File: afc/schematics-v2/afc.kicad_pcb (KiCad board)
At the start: 2 copper layers, 116.8 x 67.3 mm, 16 parts

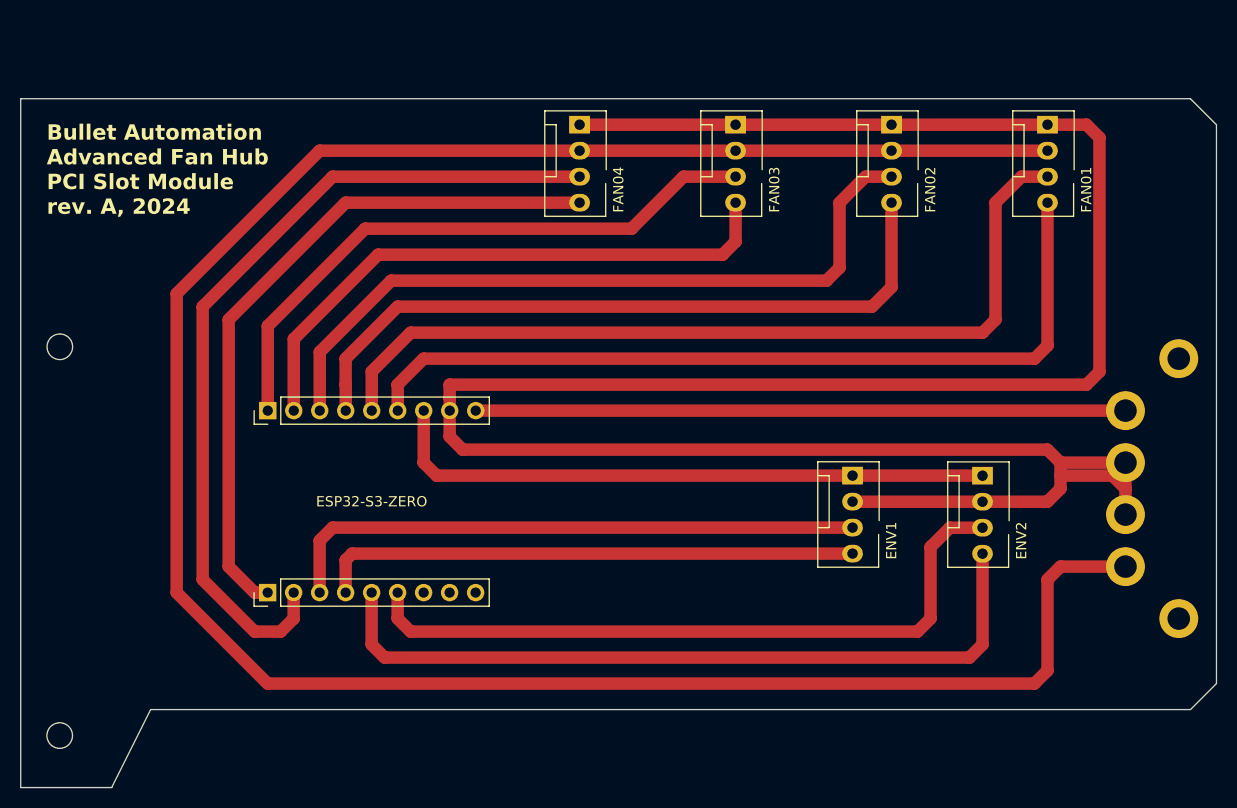
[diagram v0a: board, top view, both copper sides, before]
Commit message: adding v2 schematics
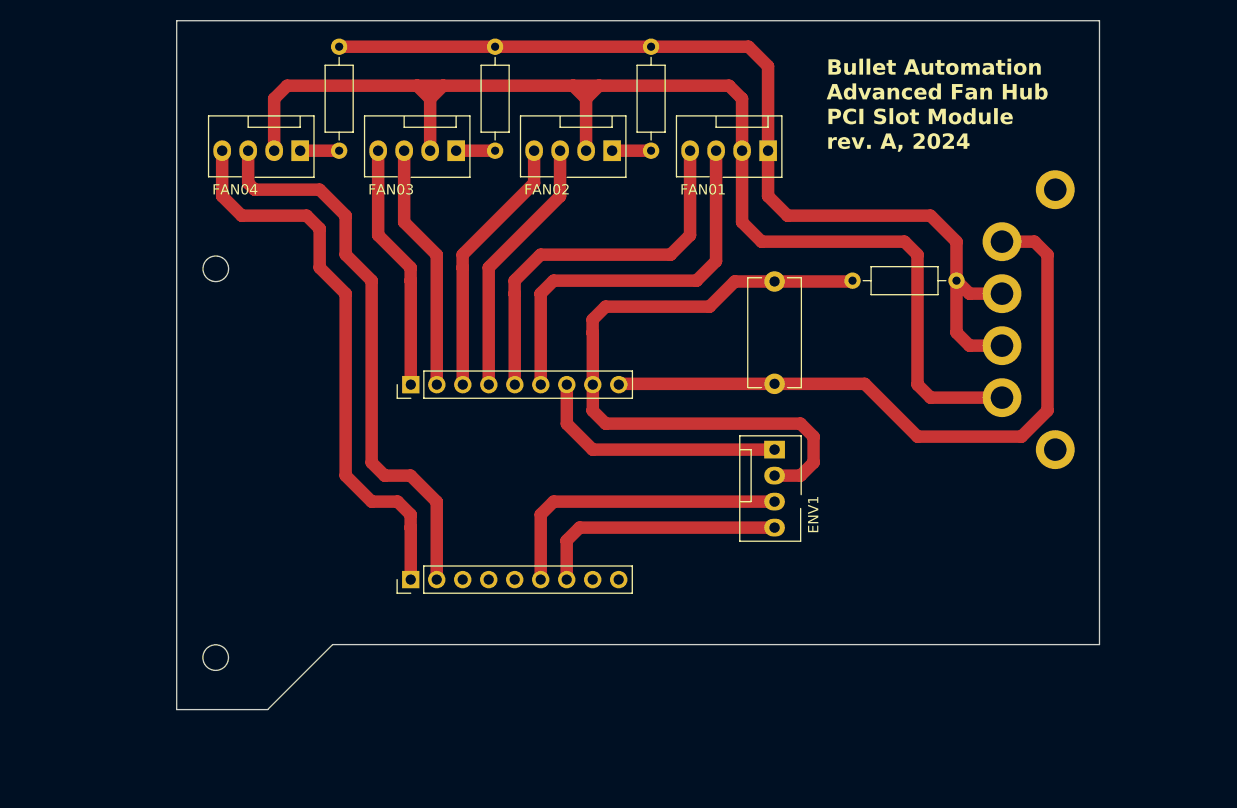
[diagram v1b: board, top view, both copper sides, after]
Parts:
- removed ENV2: FAN_H4, Connector:FanPinHeader_1x04_P2.54mm_Vertical
- added Ce: C_Disc_D10.5mm_W5.0mm_P10.00mm, Capacitor_THT:C_Disc_D10.5mm_W5.0mm_P10.00mm, F.Cu at (162.6, 87.5)
- added REF**: R_Axial_DIN0207_L6.3mm_D2.5mm_P10.16mm_Horizontal, Resistor_THT:R_Axial_DIN0207_L6.3mm_D2.5mm_P10.16mm_Horizontal, F.Cu at (135.3, 54.6)
- added REF**: R_Axial_DIN0207_L6.3mm_D2.5mm_P10.16mm_Horizontal, Resistor_THT:R_Axial_DIN0207_L6.3mm_D2.5mm_P10.16mm_Horizontal, F.Cu at (180.3, 77.5)
- added REF**: R_Axial_DIN0207_L6.3mm_D2.5mm_P10.16mm_Horizontal, Resistor_THT:R_Axial_DIN0207_L6.3mm_D2.5mm_P10.16mm_Horizontal, F.Cu at (150.5, 54.6)
- added REF**: R_Axial_DIN0207_L6.3mm_D2.5mm_P10.16mm_Horizontal, Resistor_THT:R_Axial_DIN0207_L6.3mm_D2.5mm_P10.16mm_Horizontal, F.Cu at (120.0, 54.6)
- moved FAN02 27.4 mm to (146.7, 64.8), turned to 180 degrees
- moved FAN03 27.4 mm to (131.4, 64.8), turned to 180 degrees
- moved FAN04 27.4 mm to (116.2, 64.8), turned to 180 degrees
- moved FAN01 27.4 mm to (161.9, 64.8), turned to 180 degrees
- moved ? 20.4 mm to (184.8, 73.7)
- moved ? 20.4 mm to (190.0, 68.6)
- moved ATX2 20.4 mm to (184.8, 83.8)
- moved ATX3 20.4 mm to (184.8, 78.7)
- moved ? 20.4 mm to (184.8, 88.9)
- moved ? 20.4 mm to (190.0, 94.0)
- moved ? 17.0 mm to (108.0, 114.3)
- moved PCIe_MNT_TOP 17.0 mm to (108.0, 76.3)
- moved ESP32_A 14.2 mm to (127.0, 87.6)
- moved ESP32_B 14.0 mm to (127.0, 106.7)
- moved ENV1 8.03 mm to (162.6, 94.0)
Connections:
- ESP32_A pad 1: PWM1 -> TACHO1
- ESP32_A pad 2: TACHO1 -> PWM1
- ESP32_A pad 3: PWM2 -> TACHO2
- ESP32_A pad 4: TACHO2 -> PWM2
- ESP32_A pad 5: PWM3 -> TACHO3
- ESP32_A pad 6: TACHO3 -> PWM3
- ESP32_B pad 10: SDA_1 -> (no net)
- ESP32_B pad 11: SDA_2 -> (no net)
- ESP32_B pad 12: SCL_2 -> SCL_1
- ESP32_B pad 13: (no net) -> SDA_1
- ESP32_B pad 9: SCL_1 -> (no net)
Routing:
- net 12V: track 226.4 -> 121.2 mm
- net SDA_2: track 74.7 -> 0.00 mm
- net GND: track 245.7 -> 172.7 mm
- net SCL_2: track 68.5 -> 0.00 mm
- net TACHO2: track 72.4 -> 25.8 mm
- net TACHO1: track 84.4 -> 38.2 mm
- net PWM1: track 81.6 -> 37.4 mm
- net PWM2: track 69.6 -> 25.8 mm
- net TACHO3: track 60.0 -> 24.2 mm
- net 3V3: track 60.2 -> 25.2 mm
- net PWM3: track 57.9 -> 24.2 mm
- net SDA_1: track 53.0 -> 24.7 mm
- net TACHO4: track 82.8 -> 54.7 mm
- net SCL_1: track 57.7 -> 29.7 mm
- net PWM4: track 68.0 -> 54.7 mm
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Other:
- board size 116.8 x 67.3 mm -> 90.2 x 67.3 mm
- board text removed: "ESP32-S3-ZERO"

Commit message: improvements on PCB design
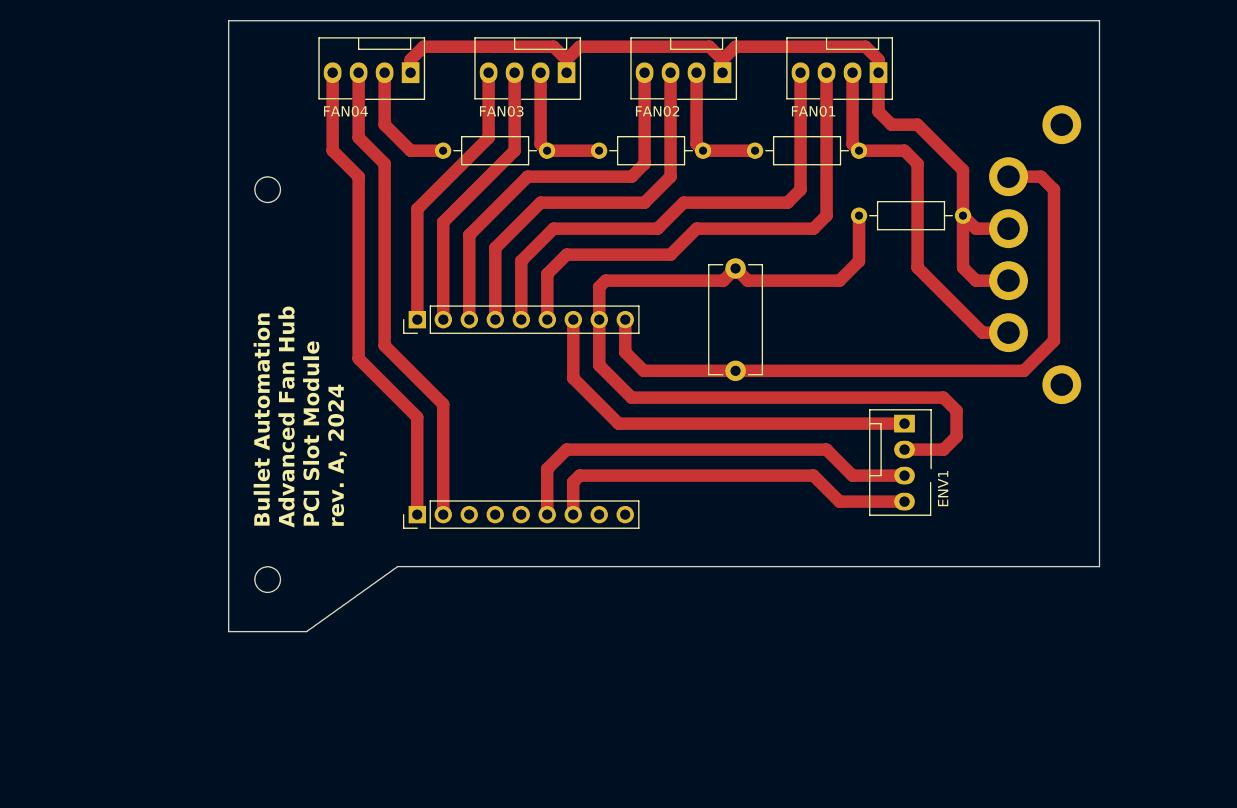
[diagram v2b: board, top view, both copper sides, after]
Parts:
- moved REF** 22.7 mm to (140.3, 64.8), turned to 180 degrees
- moved REF** 22.7 mm to (155.6, 64.8), turned to 180 degrees
- moved REF** 22.7 mm to (170.8, 64.8), turned to 180 degrees
- moved FAN03 13.2 mm to (142.2, 57.1)
- moved FAN04 13.2 mm to (127.0, 57.1)
- moved FAN01 13.2 mm to (172.7, 57.1)
- moved FAN02 13.2 mm to (157.5, 57.1)
- moved ENV1 13.0 mm to (175.3, 91.4)
- moved PCIe_MNT_TOP 9.24 mm to (113.0, 68.6)
- moved ? 9.16 mm to (113.0, 106.7)
- moved ? 6.38 mm to (190.6, 87.6)
- moved ? 6.38 mm to (185.4, 82.5)
- moved ESP32_B 6.38 mm to (127.6, 100.3)
- moved ? 6.38 mm to (190.6, 62.2)
- moved ESP32_A 6.38 mm to (127.7, 81.3)
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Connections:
- REF** pad 1: GND -> 12V (x3)
- REF** pad 2: GND -> 12V (x3)
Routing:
- net 12V: track 121.2 -> 73.6 mm
- net 3V3: track 25.2 -> 39.9 mm
- net SDA_1: track 24.7 -> 36.9 mm
- net SCL_1: track 29.7 -> 41.2 mm
- net TACHO2: track 25.8 -> 37.2 mm
- net PWM2: track 25.8 -> 37.2 mm
- net TACHO1: track 38.2 -> 48.1 mm
- net PWM1: track 37.4 -> 47.3 mm
- net TACHO4: track 54.7 -> 46.6 mm
- net PWM4: track 54.7 -> 46.6 mm
- net PWM3: track 24.2 -> 27.0 mm
- net TACHO3: track 24.2 -> 27.0 mm
- net 5V: track 65.4 -> 66.9 mm
- net GND: track 172.7 -> 173.6 mm
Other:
- board size 90.2 x 67.3 mm -> 85.1 x 59.7 mm
